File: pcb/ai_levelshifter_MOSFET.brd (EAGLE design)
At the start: 15.2 x 13.3 mm, 15 parts, among them J1 1X06, J2 1X06NOFIRST, Q1 BSS138, Q2 BSS138, Q3 BSS138, Q4 BSS138

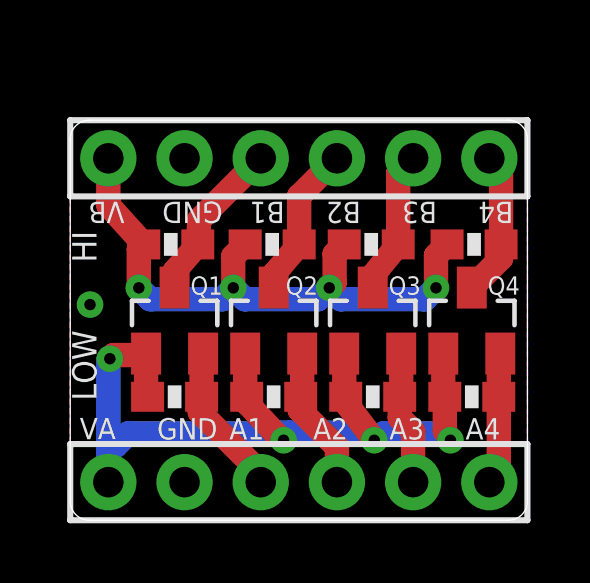
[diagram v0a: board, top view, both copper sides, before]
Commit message: updating
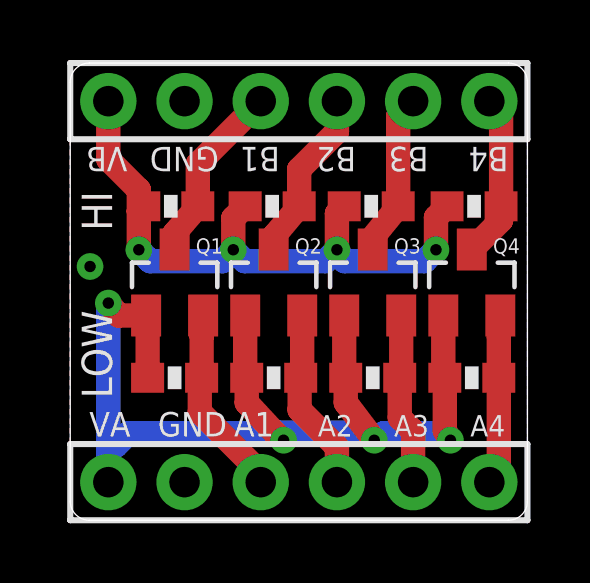
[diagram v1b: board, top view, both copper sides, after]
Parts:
- moved J2 1.91 mm to (7.62, 14.0)
- moved Q1 1.27 mm to (3.48, 7.92)
- moved Q2 1.27 mm to (6.78, 7.92)
- moved Q3 1.27 mm to (10.1, 7.92)
- moved Q4 1.27 mm to (13.4, 7.92)
- moved R2 1.27 mm to (3.35, 10.5)
- moved R4 1.27 mm to (6.73, 10.5)
- moved R6 1.27 mm to (10.0, 10.5)
- moved R8 1.27 mm to (13.5, 10.5)
- moved U$1 1.27 mm to (8.97, 9.65)
- moved R1 0.63 mm to (3.48, 4.75)
- moved R3 0.63 mm to (6.78, 4.75)
- moved R5 0.63 mm to (10.1, 4.75)
- moved R7 0.63 mm to (13.4, 4.75)
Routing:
- net VCC-A: track 28.9 -> 35.3 mm
- net A3: track 4.49 -> 5.76 mm
- net A2: track 4.84 -> 6.11 mm
- net A1: track 5.17 -> 6.42 mm
- net A4: track 4.44 -> 5.69 mm
- net VCC-B: track 20.6 -> 21.3 mm
- net B1: track 5.45 -> 6.10 mm
- net B3: track 4.84 -> 5.48 mm
- net B2: track 5.13 -> 5.77 mm
- net B4: track 4.88 -> 5.51 mm
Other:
- board size 15.2 x 13.3 mm -> 15.2 x 15.2 mm
- board text added: "v1.1"
- board text removed: "v1.0"
